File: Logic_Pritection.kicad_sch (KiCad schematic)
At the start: 16 parts

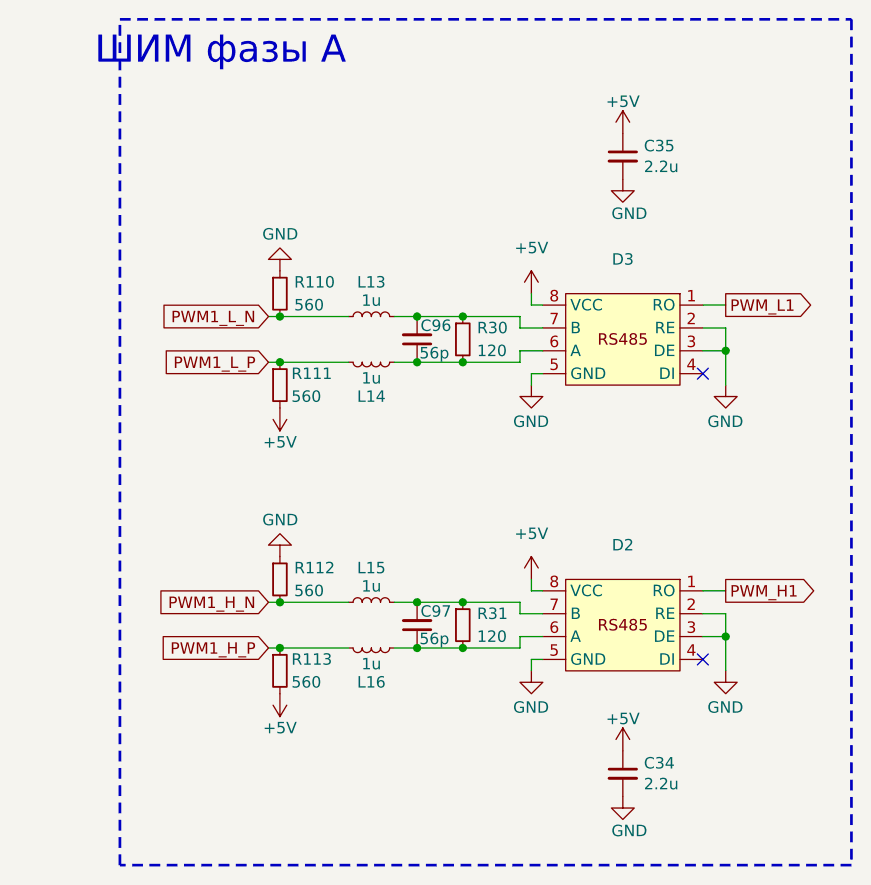
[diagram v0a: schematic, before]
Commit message: VER2.2.1: создал папку для производственных доков
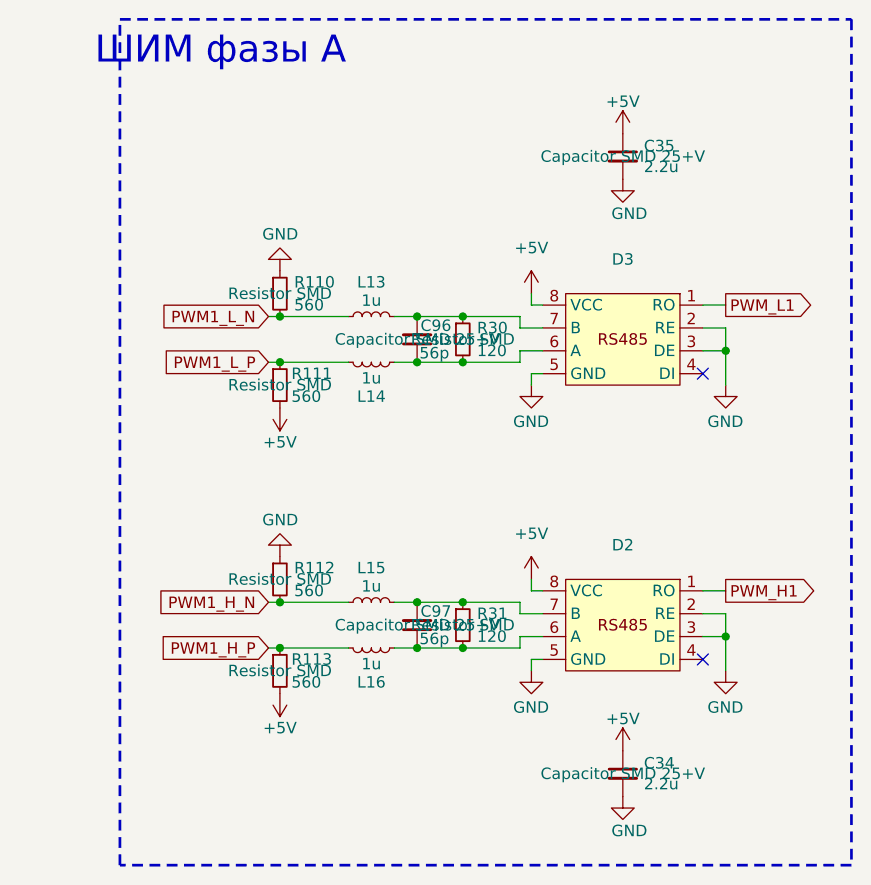
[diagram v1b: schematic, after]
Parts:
- C34, C35, C96, C97: Description P/N (none) -> Capacitor SMD 25+V
- R110, R111, R112, R113, R30, R31: Description P/N (none) -> Resistor SMD
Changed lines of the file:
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@@
 			)
 		)
-		(property "Description P/N" ""
+		(property "Description P/N" "Capacitor SMD 25+V"
 			(at 162.56 134.62 0)
 			(effects
@@
 			)
 		)
-		(property "Description P/N" ""
+		(property "Description P/N" "Resistor SMD"
 			(at 124.46 123.19 0)
 			(effects
@@
 			)
 		)
-		(property "Description P/N" ""
+		(property "Description P/N" "Resistor SMD"
 			(at 124.46 91.44 0)
 			(effects
@@
 			)
 		)
-		(property "Description P/N" ""
+		(property "Description P/N" "Capacitor SMD 25+V"
 			(at 139.7 118.11 0)
 			(effects
@@
 			)
 		)
-		(property "Description P/N" ""
+		(property "Description P/N" "Resistor SMD"
 			(at 144.78 86.36 0)
 			(effects
@@
 			)
 		)
-		(property "Description P/N" ""
+		(property "Description P/N" "Resistor SMD"
 			(at 124.46 113.03 0)
 			(effects
@@
 			)
 		)
-		(property "Description P/N" ""
+		(property "Description P/N" "Capacitor SMD 25+V"
 			(at 139.7 86.36 0)
 			(effects
@@
 			)
 		)
-		(property "Description P/N" ""
+		(property "Description P/N" "Resistor SMD"
 			(at 144.78 118.11 0)
 			(effects
@@
 			)
 		)
-		(property "Description P/N" ""
+		(property "Description P/N" "Resistor SMD"
 			(at 124.46 81.28 0)
 			(effects
@@
 			)
 		)
-		(property "Description P/N" ""
+		(property "Description P/N" "Capacitor SMD 25+V"
 			(at 162.56 66.04 0)
 			(effects
